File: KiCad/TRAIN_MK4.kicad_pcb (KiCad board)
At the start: 2 copper layers, 80 x 57 mm, 102 parts, among them J1 Screw_Terminal_01x02, J10 Conn_01x02, J11 Conn_01x02, J2 Screw_Terminal_01x02, J3 Conn_01x02, J4 Conn_01x02, J5 Conn_01x02, J6 Conn_01x02, J7 Conn_01x02, J8 Conn_01x03, J9 Conn_01x05, Q1 SUD08P06-155L, Q2 BC817W, Q3 BC817W, Q4 BC858, Q5 Q_PMOS_GSD, SW1 RotaryEncoder_Switch_MP, SW5 SW_SPDT, SW6 SW_SPDT, U1 LMR54406, U10 74AHC595, U2 KB2040, U3 MCP6001-OT, U4 MCP65R41-2402, U5 INA241A2xDDF, U6 74LVC1G240, U8 GC9A01, U9 74HC165

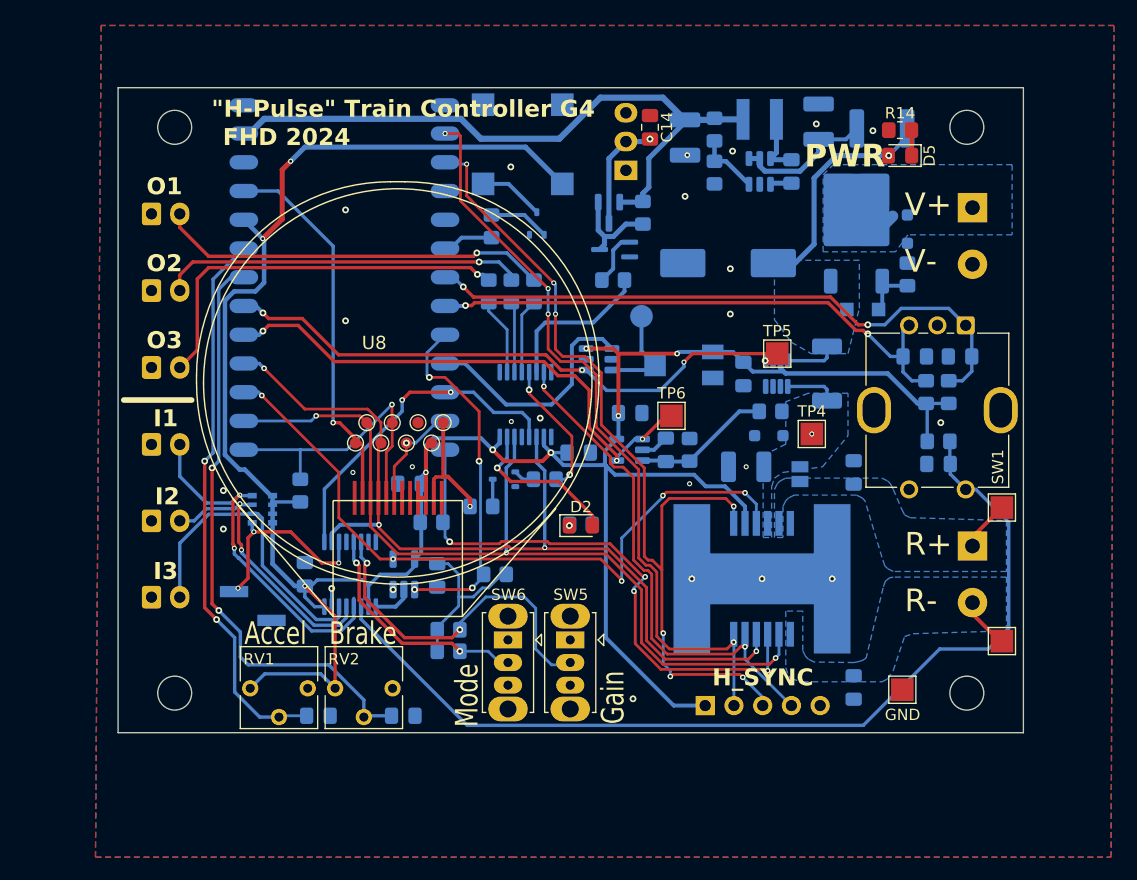
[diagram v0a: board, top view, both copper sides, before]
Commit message: Update
Dividing schematic part 1
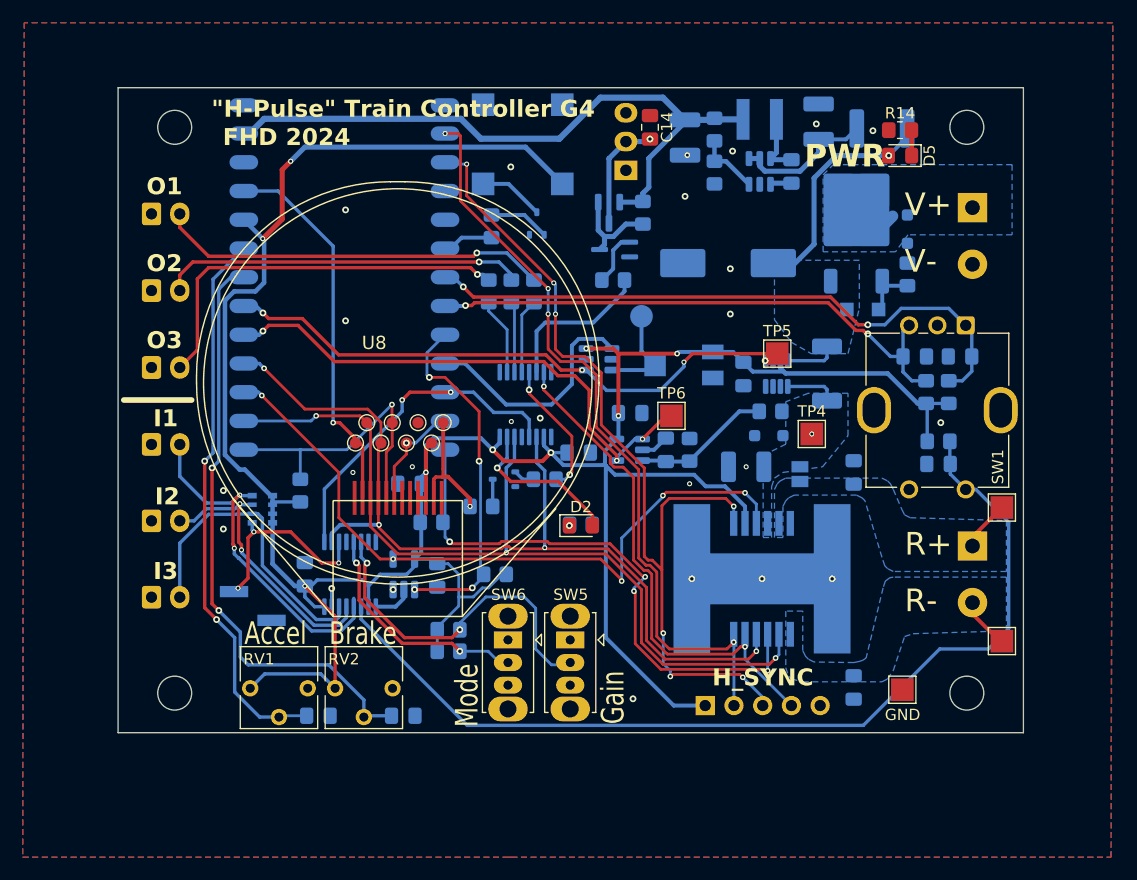
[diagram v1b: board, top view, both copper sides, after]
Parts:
- Q1: value SUD08P06-155L -> IPD85P04P407ATMA2
